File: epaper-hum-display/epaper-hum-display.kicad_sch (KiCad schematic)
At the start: 2 parts, among them U1 STM32L011

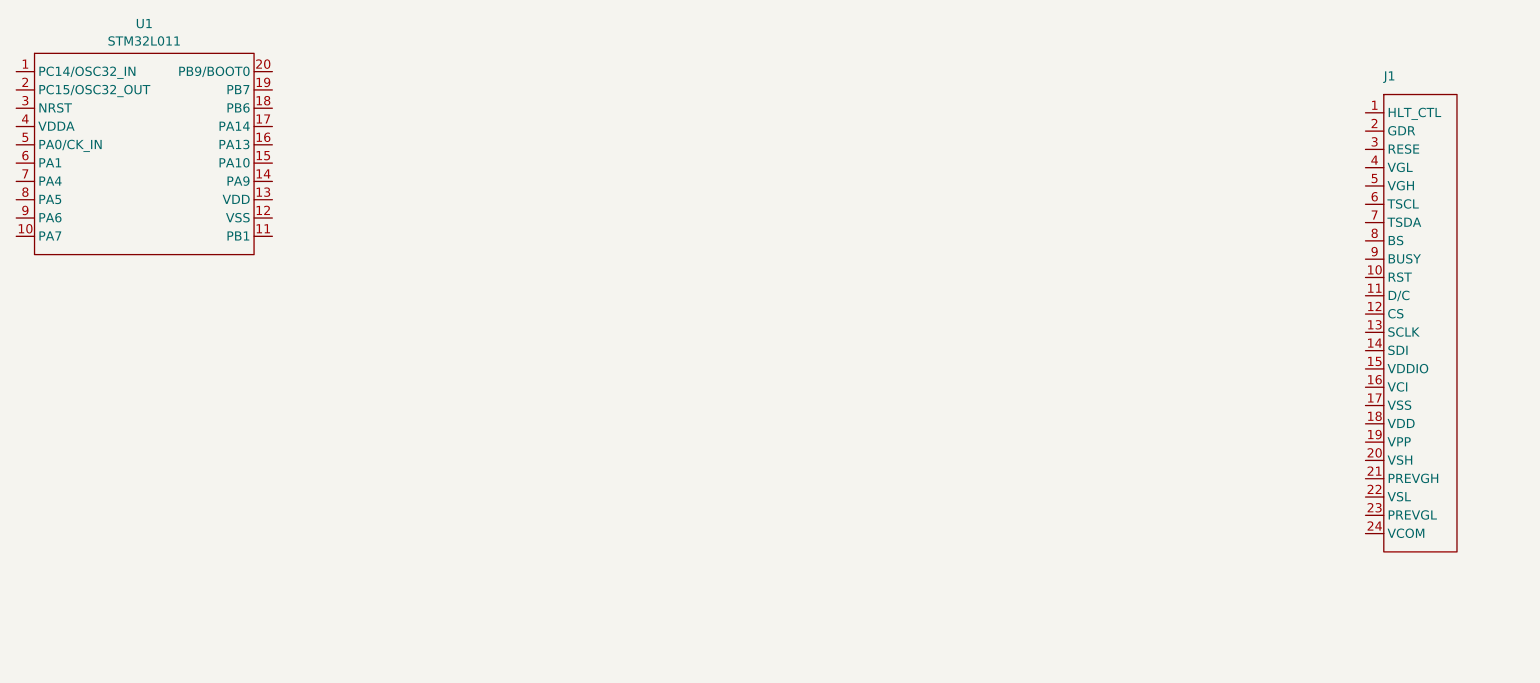
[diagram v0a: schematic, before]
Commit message: Add projects
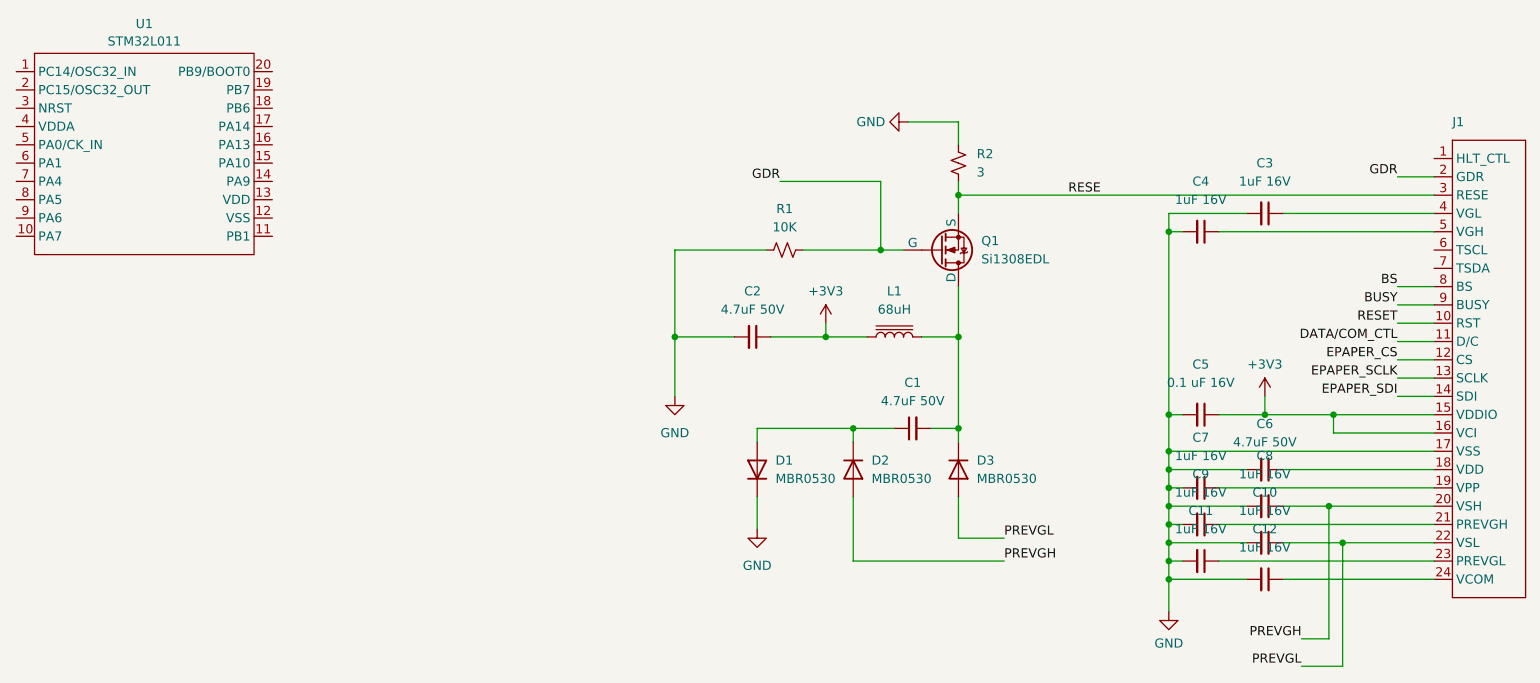
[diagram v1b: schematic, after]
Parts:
- added C1, C2, C6: 4.7uF 50V, symbol Device:C_Small
- added C10, C11, C12, C3, C4, C7, C8, C9: 1uF 16V, symbol Device:C_Small
- added C5: 0.1 uF 16V, symbol Device:C_Small
- added D1, D2, D3: MBR0530, symbol Device:D
- added L1: 68uH, symbol Device:L_Iron
- added Q1: Si1308EDL, symbol Simulation_SPICE:NMOS
- added R1: 10K, symbol Device:R_Small_US
- added R2: 3, symbol Device:R_Small_US
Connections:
- net RESET: now reaches J1.10 (RST)
- net DATA/COM_CTL: now reaches J1.11 (D/C)
- net EPAPER_CS: now reaches J1.12 (CS)
- net EPAPER_SCLK: now reaches J1.13 (SCLK)
- net EPAPER_SDI: now reaches J1.14 (SDI)
- net +3V3: now reaches J1.15 (VDDIO)
- net +3V3: now also J1.16 (VCI), C2.1, C5.1, L1.1
- net GND: now reaches J1.17 (VSS)
- net GND: now also C10.2, C11.2, C12.2, C2.2, C3.2, C4.2, C5.2, C6.2, C7.2, C8.2, C9.2, D1.1 (K), R1.1, R2.2
- net at J1.18 (VDD): now also C6.1
- net at J1.19 (VPP): now also C7.1
- net GDR: now reaches J1.2 (GDR)
- net GDR: now also Q1.2 (G), R1.2
- net PREVGH: now reaches J1.20 (VSH)
- net PREVGH: now also C8.1, D2.2 (A)
- net at J1.21 (PREVGH): now also C9.1
- net PREVGL: now reaches J1.22 (VSL)
- net PREVGL: now also C10.1, D3.2 (A)
- net at J1.23 (PREVGL): now also C11.1
- net at J1.24 (VCOM): now also C12.1
- net RESE: now reaches J1.3 (RESE)
- net RESE: now also Q1.3 (S), R2.1
- net at J1.4 (VGL): now also C3.1
- net at J1.5 (VGH): now also C4.1
- net BS: now reaches J1.8 (BS)
- net BUSY: now reaches J1.9 (BUSY)
- new net: C1.2, D3.1 (K), L1.2, Q1.1 (D)
- new net: C1.1, D1.2 (A), D2.1 (K)
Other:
- moved on the sheet: J1
